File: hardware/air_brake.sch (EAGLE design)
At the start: 18 parts

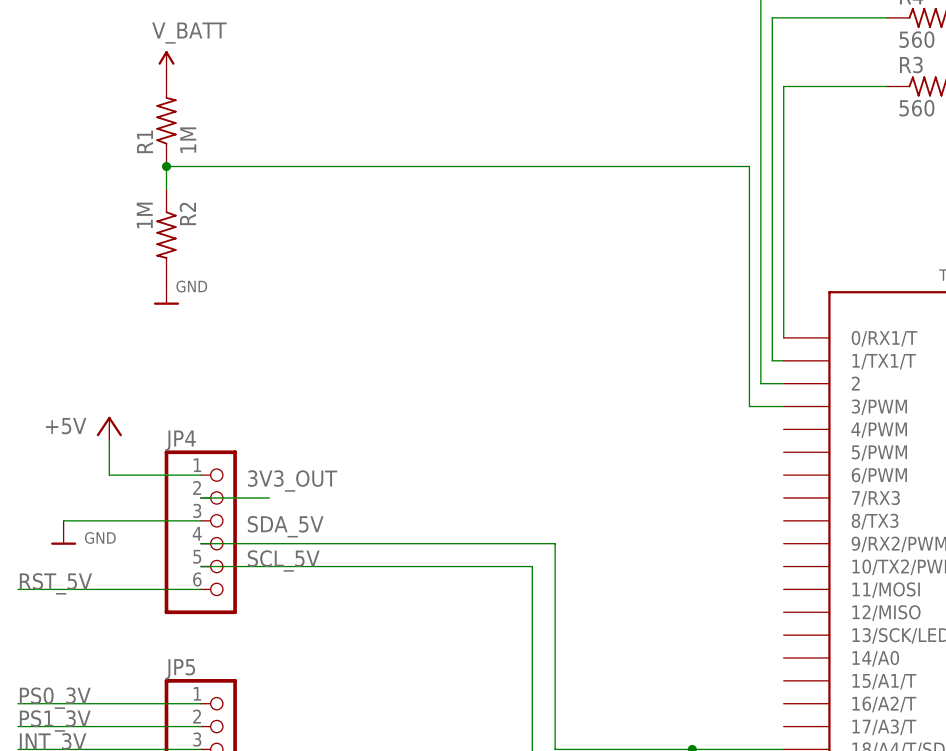
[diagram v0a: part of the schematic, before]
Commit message: very rough prelim board layout
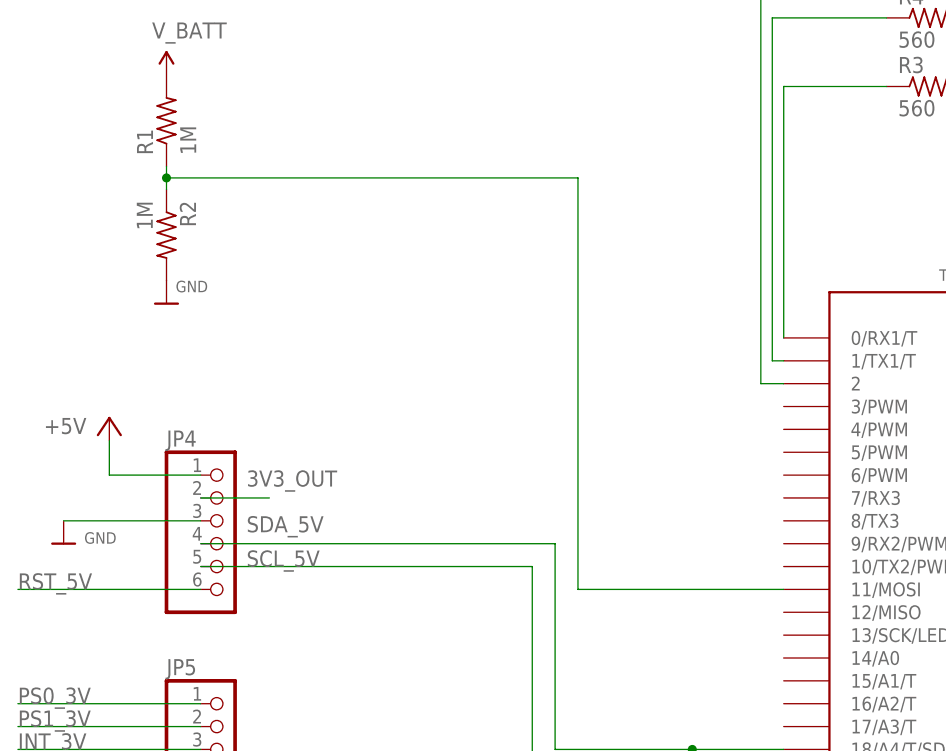
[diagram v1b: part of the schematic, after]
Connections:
- net N$1: now also TEENSY4.0.11/MOSI; no longer TEENSY4.0.3/PWM
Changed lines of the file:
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@@
 <pinref part="R2" gate="G$1" pin="1"/>
 <pinref part="R1" gate="G$1" pin="1"/>
-<wire x1="43.18" y1="128.27" x2="43.18" y2="130.81" width="0.1524" layer="91" grouprefs="BATTERY_VOLTAGE"/>
-<pinref part="TEENSY4.0" gate="G$1" pin="3/PWM"/>
-<wire x1="111.76" y1="104.14" x2="107.95" y2="104.14" width="0.1524" layer="91"/>
-<wire x1="107.95" y1="104.14" x2="107.95" y2="130.81" width="0.1524" layer="91"/>
-<wire x1="107.95" y1="130.81" x2="43.18" y2="130.81" width="0.1524" layer="91"/>
-<junction x="43.18" y="130.81"/>
+<wire x1="43.18" y1="128.27" x2="43.18" y2="129.54" width="0.1524" layer="91" grouprefs="BATTERY_VOLTAGE"/>
+<pinref part="TEENSY4.0" gate="G$1" pin="11/MOSI"/>
+<wire x1="43.18" y1="129.54" x2="43.18" y2="130.81" width="0.1524" layer="91" grouprefs="BATTERY_VOLTAGE"/>
+<wire x1="111.76" y1="83.82" x2="88.9" y2="83.82" width="0.1524" layer="91"/>
+<wire x1="88.9" y1="83.82" x2="88.9" y2="129.54" width="0.1524" layer="91"/>
+<wire x1="88.9" y1="129.54" x2="43.18" y2="129.54" width="0.1524" layer="91"/>
+<junction x="43.18" y="129.54"/>
 </segment>
 </net>
